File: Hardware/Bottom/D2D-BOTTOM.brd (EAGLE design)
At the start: 33 x 33 mm, 32 parts, among them U1 AD5242-SO16

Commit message: updated to 002
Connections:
- removed net LED.CTRL: U$4.8
- removed net PPG: C21.2, OP3.1, U1.14
- removed net TIA: C10.2, C15.1, OP4.1, U1.3
- new net A6/TIA: C10.2, C15.1, J1.5, OP4.1, U1.3
- new net A7/PPG: C21.2, J1.7, OP3.1, U1.14
- new net D29/LED.CTRL: J1.6, U$4.8
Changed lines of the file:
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@@
 <wire x1="9.5446" y1="3.929" x2="23.6982" y2="5.588" width="0" layer="19" extent="1-1"/>
 </signal>
-<signal name="TIA">
+<signal name="A6/TIA">
 <contactref element="C10" pad="2"/>
 <contactref element="U1" pad="3"/>
 <contactref element="C15" pad="1"/>
 <contactref element="OP4" pad="1"/>
+<contactref element="J1" pad="5"/>
 <wire x1="18.5166" y1="29.9584" x2="37.15" y2="24.094" width="0" layer="19" extent="1-1"/>
-<wire x1="13.3604" y1="29.3234" x2="18.5166" y2="29.9584" width="0" layer="19" extent="1-1"/>
+<wire x1="15.16" y1="33" x2="18.5166" y2="29.9584" width="0" layer="19" extent="1-1"/>
+<wire x1="13.3604" y1="29.3234" x2="15.16" y2="33" width="0" layer="19" extent="1-1"/>
 <wire x1="18.6182" y1="5.588" x2="13.3604" y2="29.3234" width="0" layer="19" extent="1-1"/>
 </signal>
@@
 <wire x1="2.7822" y1="4.1148" x2="7.5946" y2="3.929" width="0" layer="19" extent="1-1"/>
 </signal>
-<signal name="LED.CTRL">
+<signal name="D29/LED.CTRL">
 <contactref element="U$4" pad="8"/>
+<contactref element="J1" pad="6"/>
+<wire x1="7.5946" y1="6.2818" x2="17.7" y2="33" width="0" layer="19" extent="1-1"/>
 </signal>
 <signal name="N$10">
@@
 <contactref element="U1" pad="1"/>
 </signal>
-<signal name="PPG">
+<signal name="A7/PPG">
 <contactref element="U1" pad="14"/>
 <contactref element="C21" pad="2"/>
 <contactref element="OP3" pad="1"/>
-<wire x1="18.6182" y1="11.7348" x2="37.68" y2="10.16" width="0" layer="19" extent="1-1"/>
-<wire x1="14.9006" y1="26.3144" x2="18.6182" y2="11.7348" width="0" layer="19" extent="1-1"/>
+<contactref element="J1" pad="7"/>
+<wire x1="14.9006" y1="26.3144" x2="20.24" y2="33" width="0" layer="19" extent="1-1"/>
+<wire x1="18.6182" y1="11.7348" x2="14.9006" y2="26.3144" width="0" layer="19" extent="1-1"/>
+<wire x1="37.68" y1="10.16" x2="18.6182" y2="11.7348" width="0" layer="19" extent="1-1"/>
 </signal>
 <signal name="N$13">

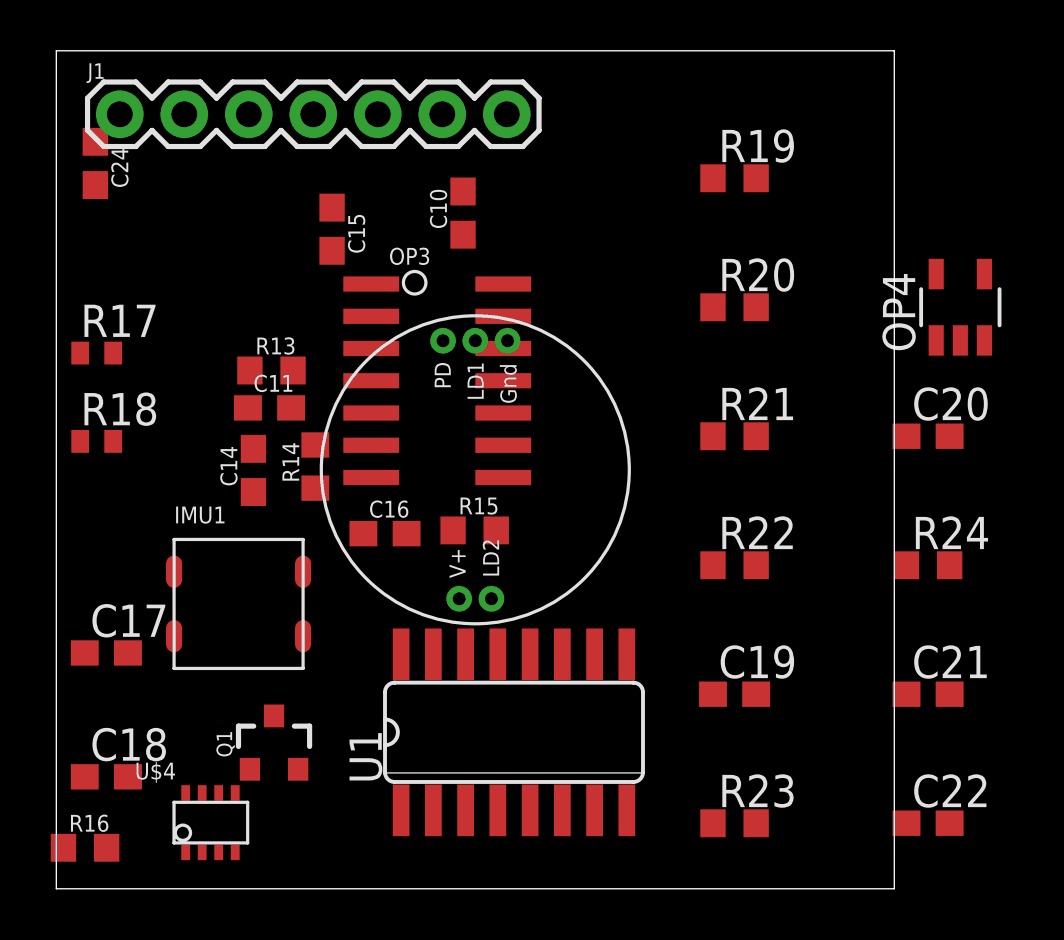
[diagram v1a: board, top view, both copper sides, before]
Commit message: checkpoint 3
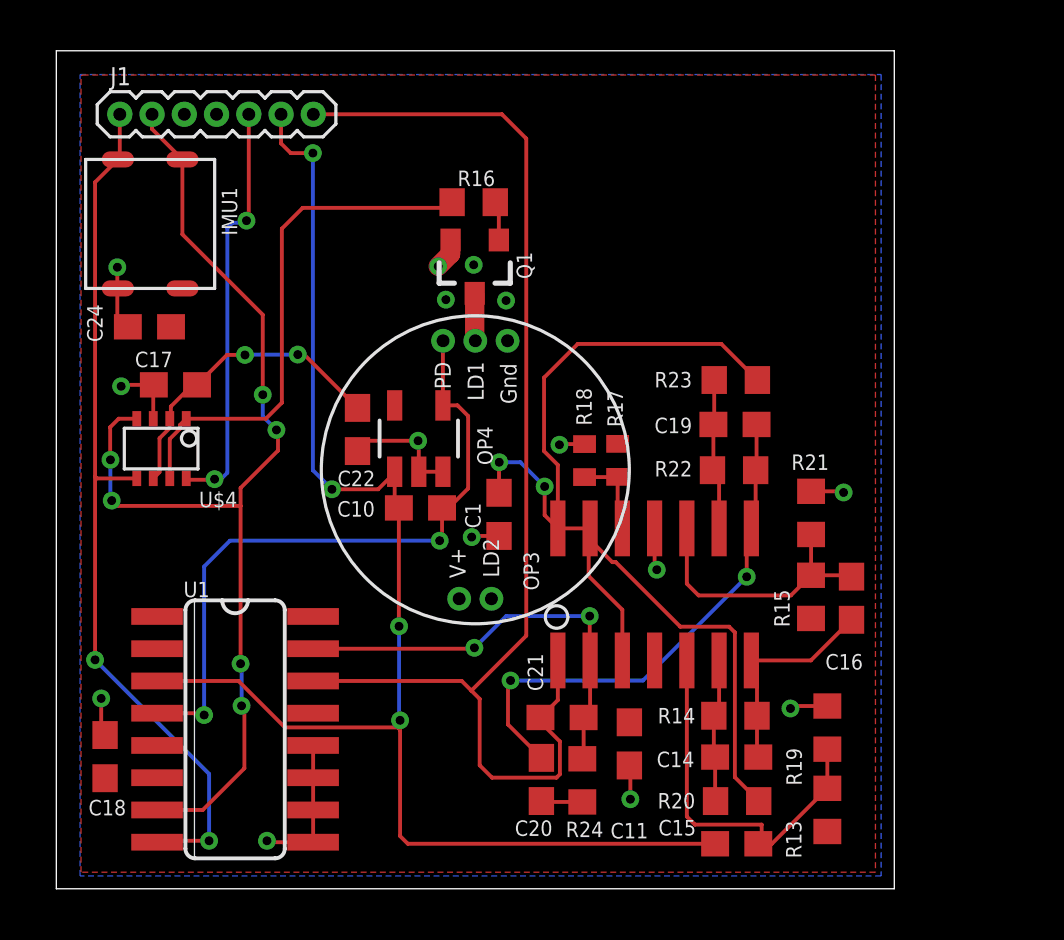
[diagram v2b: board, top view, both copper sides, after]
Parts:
- added C1: 100n, LinnesLab-Passives:C0603
- J1: device LinnesLab-Connectors:1X07 -> LinnesLab-Connectors:1X07_1.27MM
- moved R16 29.7 mm to (18.9, 29.5)
- moved C15 29.0 mm to (29.3, 4.27), turned to 0 degrees
- moved R13 27.9 mm to (32.9, 5.61), turned to 270 degrees
- moved C22 27.3 mm to (14.4, 20.6), turned to 90 degrees
- moved C14 22.1 mm to (29.3, 7.69), turned to 180 degrees
- moved OP4 21.9 mm to (16.8, 20.2)
- moved R19 21.9 mm to (32.9, 8.85), turned to 270 degrees
- moved R17 20.9 mm to (24.6, 19.4), turned to 90 degrees
- moved Q1 20.4 mm to (19.0, 27.0), turned to 180 degrees
- moved C20 20.4 mm to (21.6, 6.80), turned to 270 degrees
- moved R20 19.4 mm to (29.3, 5.95), turned to 180 degrees
- moved C11 19.4 mm to (25.1, 8.21), turned to 90 degrees
- moved R14 19.2 mm to (29.2, 9.31), turned to 0 degrees
- moved R18 19.2 mm to (23.3, 19.4), turned to 270 degrees
- moved C16 18.5 mm to (33.8, 13.9), turned to 90 degrees
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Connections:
- removed net LED: Q1.3
- net 3.3V: now also J1.4
- net A6/TIA: now also J1.6; no longer J1.5
- net D29/LED.CTRL: now also J1.5; no longer J1.6
- net GND: now also C1.1, J1.3
- net LED.C: now also Q1.3
- net SCL: now also J1.2
- net SDA: now also J1.1
- net VREF: now also C1.2
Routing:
- net A6/TIA: track 0.00 -> 56.2 mm, vias 0 -> 4
- net A7/PPG: track 0.00 -> 49.4 mm
- net VREF: track 0.00 -> 42.6 mm, vias 0 -> 2
- net SCL: track 0.00 -> 41.9 mm, vias 0 -> 6
- net SDA: track 0.00 -> 34.6 mm, vias 0 -> 2
- net PD.C: track 0.00 -> 26.7 mm, vias 0 -> 2
- net GND: track 0.00 -> 26.2 mm, vias 0 -> 15
- net N$19: track 0.00 -> 21.0 mm, vias 0 -> 2
- net N$9: track 0.00 -> 20.6 mm
- net G.W2: track 0.00 -> 17.4 mm, vias 0 -> 2
- net D29/LED.CTRL: track 0.00 -> 16.5 mm, vias 0 -> 2
- net N$13: track 0.00 -> 15.2 mm
- net 3.3V: track 0.00 -> 12.2 mm, vias 0 -> 2
- net N$17: track 0.00 -> 10.8 mm
- net N$16: track 0.00 -> 8.53 mm
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- added copper zone on layer 1, net 3.3V
- added copper zone on layer 16, net GND
